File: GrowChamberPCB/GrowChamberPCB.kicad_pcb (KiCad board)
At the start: 4 copper layers, 100 x 100 mm, 194 parts, among them J1 Mister, J10 FoggerBasin, J11 TP, J12 Moisture Sensor 3, J13 Moisture Sensor 2, J14 UART, J15 FAE Fan, J16 DrainLevel, J17 TP, J18 TP, J19 TP, J2 Moisture Sensor 1, J20 TP, J21 TP, J22 TP, J23 TP, J24 TP, J25 TP, J26 TP, J27 TP, J28 TP, J29 TP, J3 SCD30, J30 TP, J31 TP, J32 TP, J33 TP, J34 TP, J35 TP, J36 TP, J37 TP, J38 TP, J39 TP, J4 Heater Fans, J40 TP, J41 TP, J42 TP, J43 TP, J44 TP, J45 TP, J47 Conn_01x04, J48 Conn_01x09, J49 TP, J5 Fogger Solenoid, J50 TP, J51 TP, J52 TP, J53 TP, J6 Drain Solenoid, J7 Water Solenoid, J8 Glycol Solenoid, J9 CircFan, P1 12V_In, P2 120V, P3 Screw Terminal, Q1 MOSFET, Q10 NPN, Q11 MOSFET, Q12 NPN, Q13 MOSFET, Q15 NPN, Q17 NPN, Q18 MOSFET, Q2 NPN, Q3 MOSFET, Q4 NPN, Q5 MOSFET, Q6 NPN, Q7 MOSFET, Q8 BRT30N70P3, Q9 NPN, SW1 Reset_Button_Internal, SW2 ResetButton_External, SW3 Bootmode_Internal, SW4 BootMode_External, U10 1N4007W, U11 AP63203WU-7, U12 1N4007W, U13 1N4007W, U14 1N4007W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

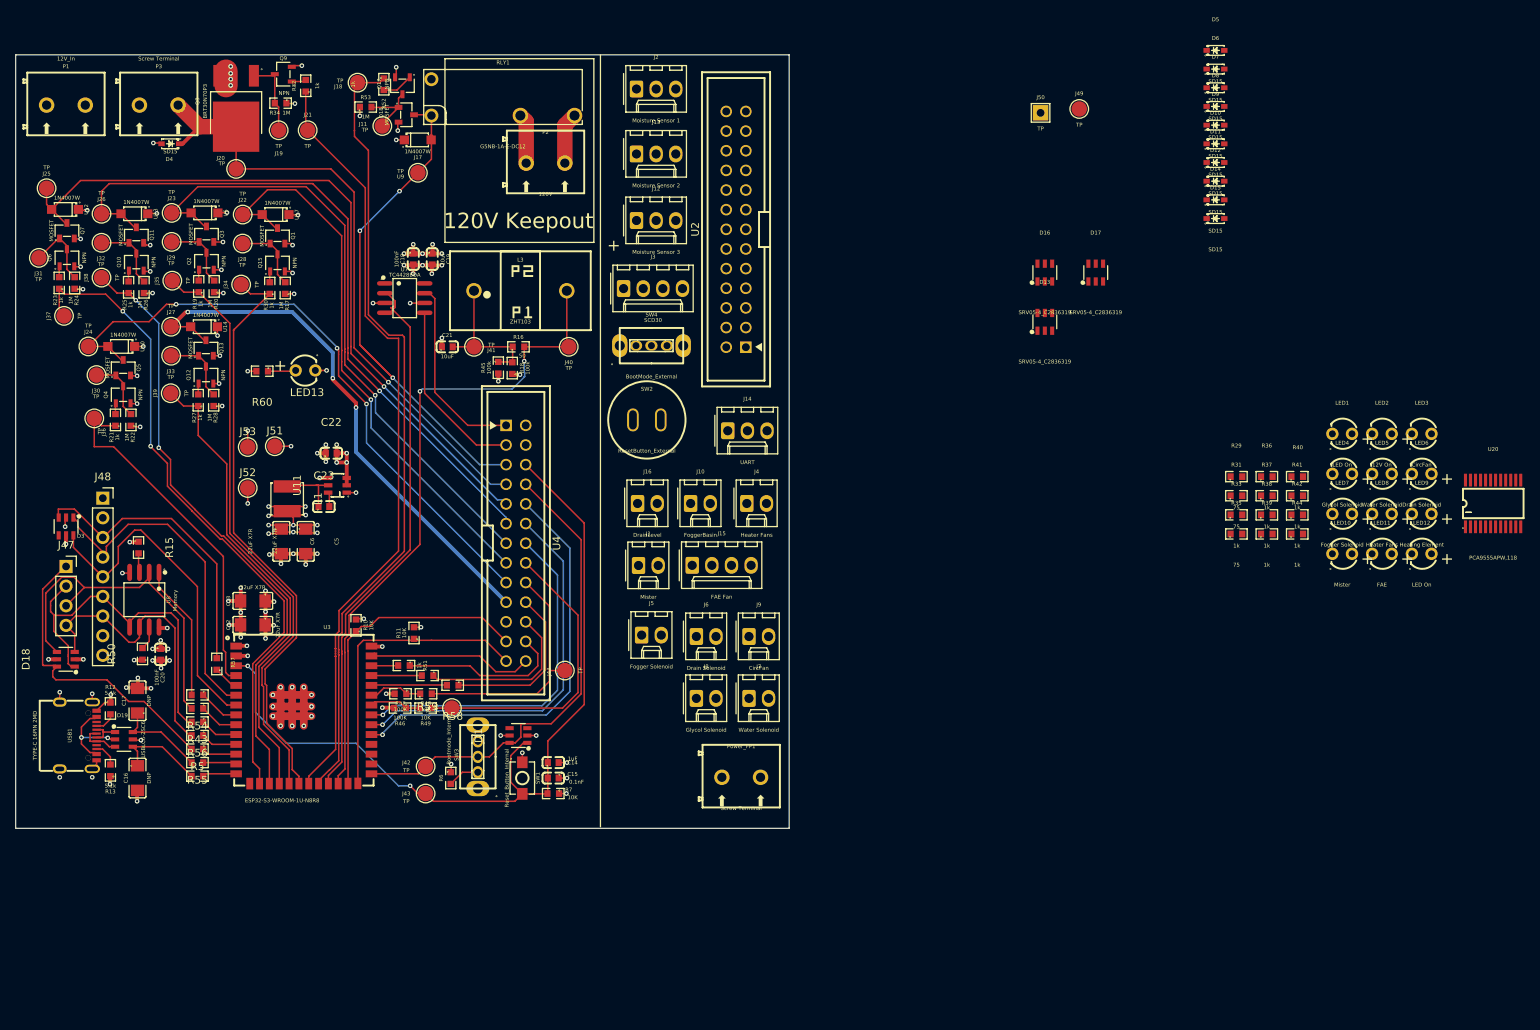
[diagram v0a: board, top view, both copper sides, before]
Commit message: finished routing
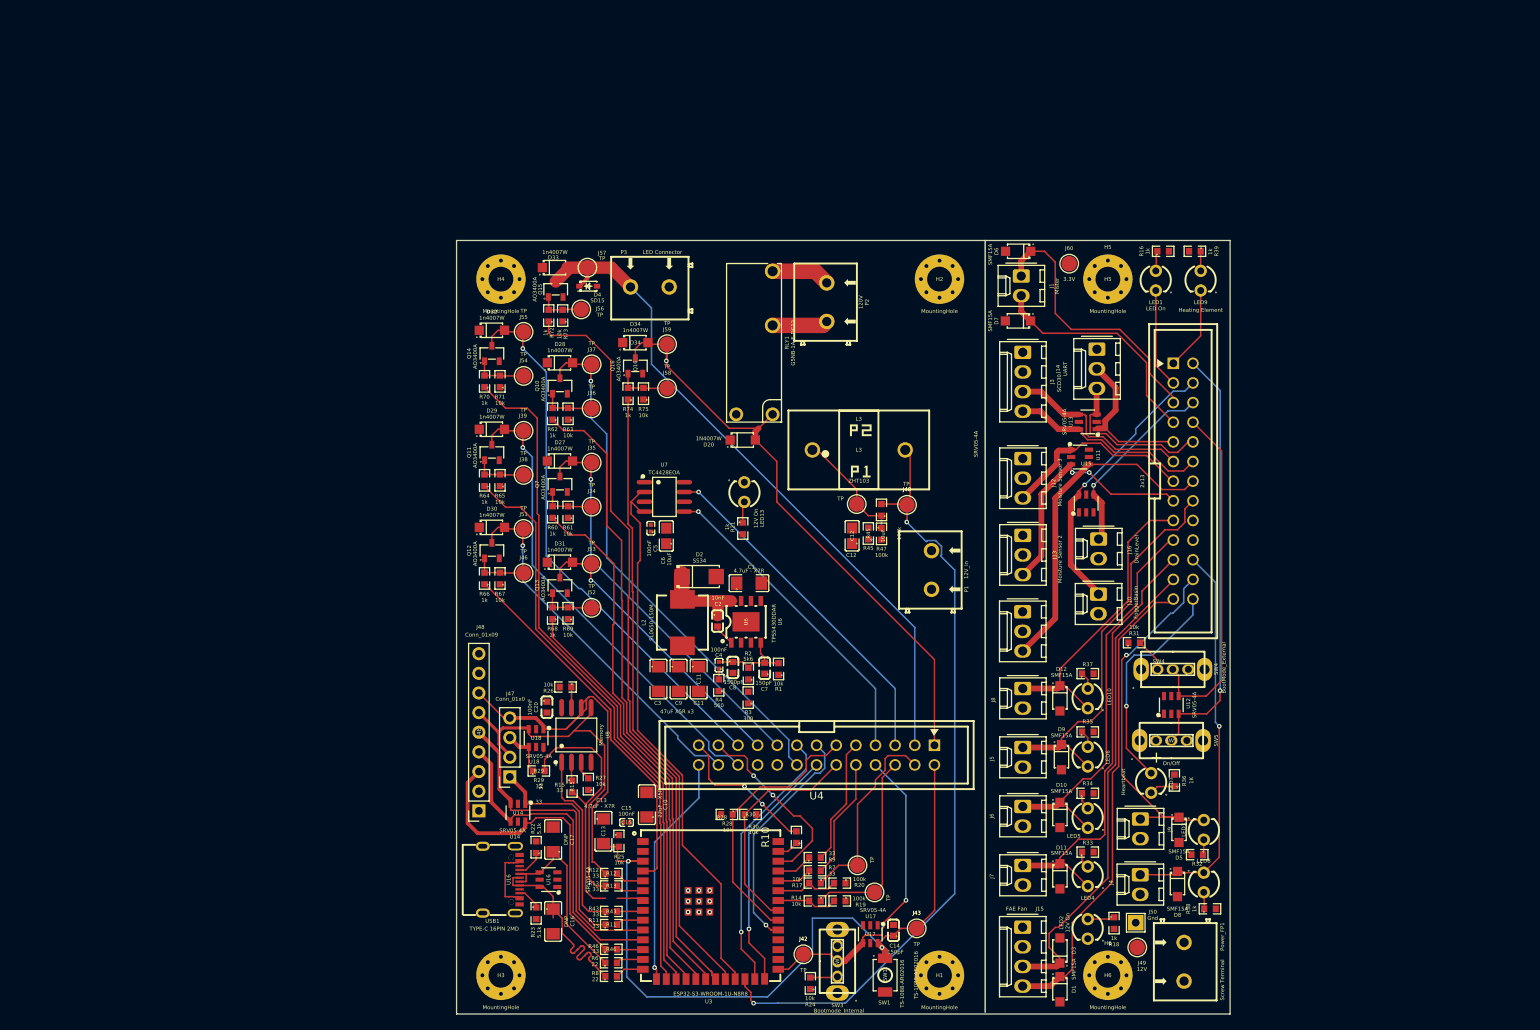
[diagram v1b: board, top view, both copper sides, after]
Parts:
- removed C18, C23: 100nF, easyeda2kicad:C0603
- removed C19, C21, C22: 10uF, easyeda2kicad:C0603
- removed D13, D16, D17, D18: SRV05-4_C2836319, easyeda2kicad:SOT-23-6_L2.9-W1.6-P0.95-LS2.8-BL
- removed D14, D15: SD15, easyeda2kicad:SOD-323_L1.7-W1.3-LS2.6-RD
- removed D19: USBLC6-2SC6, easyeda2kicad:SOT-23-6_L2.9-W1.6-P0.95-LS2.8-BL
- removed J11, J17, J18, J19, J20, J21, J22, J23, J24, J25, J26, J27, J28, J29, J30, J31, J32, J33: TP, TestPoint:TestPoint_Pad_D2.0mm
- removed L1: ANR4030T3R9M, easyeda2kicad:IND-SMD_L4.0-W4.0
- removed LED11: FAE, easyeda2kicad:LED-TH_BD3.9-P2.54-RD_RED
- removed LED12: LED On, easyeda2kicad:LED-TH_BD3.9-P2.54-RD_RED
- removed Q1, Q18, Q3, Q5: MOSFET, easyeda2kicad:SOT-23-3_L2.9-W1.3-P1.90-LS2.4-BR
- removed Q17, Q2, Q4, Q6, Q9: NPN, easyeda2kicad:SOT-23-3_L3.0-W1.7-P0.95-LS2.9-BR
- removed Q8: BRT30N70P3, easyeda2kicad:TO-252-2_L6.6-W6.1-P4.60-LS10.0-BR-CW
- removed R40, R41, R42, R44, R51, R52: 1k, easyeda2kicad:R0603
- removed R48, R49, R50: 10K, easyeda2kicad:R0603
- removed R53: 1M, easyeda2kicad:R0603
- removed R54, R55, R56, R57, R58, R59: 33, easyeda2kicad:R0603
- removed SW2: ResetButton_External, easyeda2kicad:CONN-TH_PB-05B-R
- removed U10, U5, U9: 1N4007W, easyeda2kicad:SOD-123FL_L2.7-W1.8-LS3.7-RD
- removed U20: PCA9555APW,118, easyeda2kicad:TSSOP-24_L7.8-W4.4-P0.65-LS6.4-BL
- added C1: 4.7uF - X7R, easyeda2kicad:C1206, F.Cu at (106.8, 80.3)
- added C10: 22uF - X5R, easyeda2kicad:C1206, F.Cu at (93.6, 108.9)
- added C11: 47uF X5R, easyeda2kicad:C1206, F.Cu at (100.3, 92.7)
- added C2: 10nF, easyeda2kicad:C0603, F.Cu at (102.7, 85.2)
- added C3: 47uF X5R, easyeda2kicad:C1206, F.Cu at (95.1, 92.7)
- added C4: 100nF, easyeda2kicad:C0402, F.Cu at (102.9, 90.9)
- added C7: 150pF, easyeda2kicad:C0603, F.Cu at (108.8, 91.3)
- added C8: 1500pF, easyeda2kicad:C0603, F.Cu at (104.7, 91.2)
- added C9: 47uF X5R, easyeda2kicad:C1206, F.Cu at (97.7, 92.7)
- added D2: SS34, easyeda2kicad:SMA_L4.3-W2.6-LS5.2-RD, F.Cu at (100.4, 79.5)
- added D20: 1N4007W, easyeda2kicad:SOD-123FL_L2.7-W1.8-LS3.8-RD, F.Cu at (106.0, 61.8)
- added D27: 1n4007W, easyeda2kicad:SOD-123FL_L2.7-W1.8-LS3.8-RD, F.Cu at (82.4, 64.5)
- added D28: 1n4007W, easyeda2kicad:SOD-123FL_L2.7-W1.8-LS3.8-RD, F.Cu at (82.4, 51.8)
- added D29: 1n4007W, easyeda2kicad:SOD-123FL_L2.7-W1.8-LS3.8-RD, F.Cu at (73.6, 60.4)
- added D30: 1n4007W, easyeda2kicad:SOD-123FL_L2.7-W1.8-LS3.8-RD, F.Cu at (73.6, 73.1)
- added D31: 1n4007W, easyeda2kicad:SOD-123FL_L2.7-W1.8-LS3.8-RD, F.Cu at (82.4, 77.6)
- added D32: 1n4007W, easyeda2kicad:SOD-123FL_L2.7-W1.8-LS3.8-RD, F.Cu at (73.6, 47.6)
- added D33: 1n4007W, easyeda2kicad:SOD-123FL_L2.7-W1.8-LS3.8-RD, F.Cu at (81.7, 39.5)
- added D34: 1n4007W, easyeda2kicad:SOD-123FL_L2.7-W1.8-LS3.8-RD, F.Cu at (92.1, 49.2)
- added H1: MountingHole, MountingHole:MountingHole_3.2mm_M3_Pad_Via, F.Cu at (131.4, 131.0)
- added H2: MountingHole, MountingHole:MountingHole_3.2mm_M3_Pad_Via, F.Cu at (131.4, 41.0)
- added H3: MountingHole, MountingHole:MountingHole_3.2mm_M3_Pad_Via, F.Cu at (74.7, 131.0)
- added H4: MountingHole, MountingHole:MountingHole_3.2mm_M3_Pad_Via, F.Cu at (74.7, 41.0)
- added H5: MountingHole, MountingHole:MountingHole_3.2mm_M3_Pad_Via, F.Cu at (153.2, 41.0)
- added H6: MountingHole, MountingHole:MountingHole_3.2mm_M3_Pad_Via, F.Cu at (153.2, 131.0)
- added J46: TP, TestPoint:TestPoint_Pad_D2.0mm, F.Cu at (77.7, 79.0)
- added J54: TP, TestPoint:TestPoint_Pad_D2.0mm, F.Cu at (77.7, 53.5)
- added J55: TP, TestPoint:TestPoint_Pad_D2.0mm, F.Cu at (77.7, 47.8)
- added J56: TP, TestPoint:TestPoint_Pad_D2.0mm, F.Cu at (85.1, 44.9)
- added J57: TP, TestPoint:TestPoint_Pad_D2.0mm, F.Cu at (85.9, 39.5)
- added J58: TP, TestPoint:TestPoint_Pad_D2.0mm, F.Cu at (96.2, 55.1)
- added J59: TP, TestPoint:TestPoint_Pad_D2.0mm, F.Cu at (96.2, 49.4)
- added J60: TP, TestPoint:TestPoint_Pad_D2.0mm, F.Cu at (148.2, 39.0)
- added L2: SL0650-150M, easyeda2kicad:IND-SMD_L7.0-W6.6, F.Cu at (98.2, 85.4)
- added Q14: AO3400A, easyeda2kicad:SOT-23-3_L2.9-W1.3-P1.90-LS2.4-BR, F.Cu at (73.6, 50.6)
- added Q16: AO3400A, easyeda2kicad:SOT-23-3_L2.9-W1.3-P1.90-LS2.4-BR, F.Cu at (92.1, 52.2)
- added R1: 10k, easyeda2kicad:R0603, F.Cu at (110.6, 91.4)
- added R14: 10k, easyeda2kicad:R0603, F.Cu at (115.3, 121.4)
- added R2: 5k6, easyeda2kicad:R0603, F.Cu at (106.7, 92.0)
- added R3: 300, easyeda2kicad:R0603, F.Cu at (106.7, 95.1)
- added R4: 560, easyeda2kicad:R0603, F.Cu at (102.9, 93.5)
- added R61: 10k, easyeda2kicad:R0603, F.Cu at (83.4, 71.1)
- added R62: 1k, easyeda2kicad:R0603, F.Cu at (81.4, 58.4)
- added R63: 10k, easyeda2kicad:R0603, F.Cu at (83.4, 58.4)
- added R64: 1k, easyeda2kicad:R0603, F.Cu at (72.6, 67.0)
- added R65: 10k, easyeda2kicad:R0603, F.Cu at (74.6, 67.0)
- added R66: 1k, easyeda2kicad:R0603, F.Cu at (72.6, 79.7)
- added R67: 10k, easyeda2kicad:R0603, F.Cu at (74.6, 79.7)
- added R68: 1k, easyeda2kicad:R0603, F.Cu at (81.4, 84.2)
- added R69: 10k, easyeda2kicad:R0603, F.Cu at (83.4, 84.2)
- added R70: 1k, easyeda2kicad:R0603, F.Cu at (72.6, 54.2)
- added R71: 10k, easyeda2kicad:R0603, F.Cu at (74.6, 54.2)
- added R72: 1k, easyeda2kicad:R0603, F.Cu at (80.9, 45.7)
- added R73: 10k, easyeda2kicad:R0603, F.Cu at (82.7, 45.7)
- added R74: 1k, easyeda2kicad:R0603, F.Cu at (91.2, 55.8)
- added R75: 10k, easyeda2kicad:R0603, F.Cu at (93.2, 55.8)
- added SW5: On/Off, easyeda2kicad:SW-TH_SS-12D02-VG4, F.Cu at (161.4, 100.7)
- added U15: SRV05-4A, easyeda2kicad:SOT-23-6_L2.9-W1.6-P0.95-LS2.9-BL, F.Cu at (150.4, 70.0)
- added U16: SRV05-4A, easyeda2kicad:SOT-23-6_L2.9-W1.6-P0.95-LS2.9-BL, F.Cu at (80.9, 118.6)
- added U18: SRV05-4A, easyeda2kicad:SOT-23-6_L2.9-W1.6-P0.95-LS2.9-BL, F.Cu at (79.3, 100.3)
- added U6: TPS5430DDAR, easyeda2kicad:ESOP-8_L4.9-W3.9-P1.27-LS6.0-TL-EP, F.Cu at (106.4, 85.3)
- C12, C6: value 22uF X7R -> 10uF; footprint easyeda2kicad:C1206 -> easyeda2kicad:C0805
- C13: value 22uF X7R -> 4.7uF - X7R
- C14: value 1uF -> 150pF
- C15: value 0.1nF -> 100nF; footprint easyeda2kicad:C0603 -> easyeda2kicad:C0402
- C5: value 22uF X7R -> 100nF; footprint easyeda2kicad:C1206 -> easyeda2kicad:C0402
- D1, D3: value SRV05-4_C2836319 -> SMF15A; footprint easyeda2kicad:SOT-23-6_L2.9-W1.6-P0.95-LS2.8-BL -> easyeda2kicad:SOD-123FL_L2.7-W1.8-LS3.8-RD
- D10, D11, D12, D5, D6, D7, D8, D9: value SD15 -> SMF15A; footprint easyeda2kicad:SOD-323_L1.7-W1.3-LS2.6-RD -> easyeda2kicad:SOD-123FL_L2.7-W1.8-LS3.8-RD
- J49: value TP -> 12V
- J50: value TP -> Gnd
- LED10: value Mister -> 12V On
- LED4: value Glycol Solenoid -> 12V On
- LED5: value Water Solenoid -> 12V On
- LED6: value Drain Solenoid -> 12V On
- LED7: value Fogger Solenoid -> 12V On
- P3: value Screw Terminal -> LED Connector
- Q10, Q12, Q15: value NPN -> AO3400A; footprint easyeda2kicad:SOT-23-3_L3.0-W1.7-P0.95-LS2.9-BR -> easyeda2kicad:SOT-23-3_L2.9-W1.3-P1.90-LS2.4-BR
- Q11, Q13, Q7: value MOSFET -> AO3400A
- R10: value 10K -> 1k
- R11, R15, R7: value 10K -> 33
- R12, R13: value 5.1k -> 33
- R16: value 50 -> 1k
- R17, R24, R26, R28: value 1M -> 10k
- R18: value 100k -> 1k
- R19: value 1k -> 100k
- R20: value 1M -> 100k
- R22: value 1M -> 5.1k
- R23: value 1k -> 5.1k
- R25, R27, R30: value 1k -> 10k
- R29: value 75 -> 33
- R31: value 75 -> 10k
- R34: value 1M -> 1k
- R35: value 75 -> 1k
- R36: value 1k -> 0603WAF750JT5E
- R46: value 100K -> 33
- R47: value 100K -> 100k
- R5: value 33 -> 50
- R6: value 10K -> 22
- R9: value 22 -> 33
- SW1: value Reset_Button_Internal -> TS-1088-AR02016; footprint easyeda2kicad:SW-SMD_L4.0-W2.9-LS5.0 -> easyeda2kicad:SW-SMD_L3.9-W3.0-P4.45
- U11: value AP63203WU-7 -> SRV05-4A; footprint easyeda2kicad:TSOT-26_L2.9-W1.6-P0.95-LS2.8-BL -> easyeda2kicad:SOT-23-6_L2.9-W1.6-P0.95-LS2.9-BL
- U12, U13, U14, U17: value 1N4007W -> SRV05-4A; footprint easyeda2kicad:SOD-123FL_L2.7-W1.8-LS3.7-RD -> easyeda2kicad:SOT-23-6_L2.9-W1.6-P0.95-LS2.9-BL
- U2: value ZX-IDC2.54-2-13PZZ -> 2x13
- moved U12 156.7 mm to (161.4, 96.0), turned to 0 degrees
- moved R32 152.2 mm to (164.8, 115.4), turned to 180 degrees
- moved D3 139.7 mm to (147.0, 127.8), turned to 90 degrees
- moved R34 137.3 mm to (150.6, 107.5), turned to 0 degrees
- moved R24 131.3 mm to (114.7, 132.0)
- moved P1 127.0 mm to (130.4, 78.6), turned to 90 degrees
- moved U13 126.2 mm to (150.6, 59.5), turned to 90 degrees
- moved U17 120.7 mm to (122.5, 125.7)
- moved R19 114.8 mm to (118.5, 121.4), turned to 180 degrees
- moved R20 111.8 mm to (118.5, 119.1), turned to 180 degrees
- moved J49 108.7 mm to (157.0, 127.4), turned to 180 degrees
- moved R18 105.8 mm to (154.0, 124.2), turned to -90 degrees
- moved J50 105.4 mm to (156.8, 124.2), turned to -90 degrees
- moved R17 103.0 mm to (115.3, 119.1), turned to 180 degrees
- moved R23 102.2 mm to (79.3, 123.0), turned to -90 degrees
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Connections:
- C12 pad 2: 3.3V -> Net-(J41-Pin_1)
- C13 pad 2: 3.3V -> EN
- C15 pad 1: GND -> 3.3V
- C15 pad 2: EN -> GND
- C16 pad 1: Out_D+ -> D+
- C17 pad 1: Out_D- -> D-
- C5 pad 1: 3.3V -> GND
- C5 pad 2: GND -> 12V
- C6 pad 1: 3.3V -> GND
- C6 pad 2: GND -> 12V
- D1 pad 1: EN -> External_Fan_PWM_FP
- D1 pad 2: GND -> GND_FP
- D10 pad 1: WaterSol_FP -> DrainSol_FP
- D11 pad 1: GlycolSol_FP -> FoggerSol_FP
- D12 pad 1: Piezo1_FP -> GlycolSol_FP
- D3 pad 1: Display_Reset -> Fan_Tach_FP
- D3 pad 2: GND -> GND_FP
- D7 pad 1: Heater Fans_FP -> Piezo1_FP
- D8 pad 1: FoggerSol_FP -> Heater Fans_FP
- D9 pad 1: DrainSol_FP -> WaterSol_FP
- J1 pad 1: Piezo1_FP -> Piezo2_FP
- J1 pad 2: Piezo2_FP -> Piezo1_FP
- J16 pad 1: 3.3V_FP -> Drain_Level_FP
- J16 pad 2: Drain_Level_FP -> 3.3V_FP
- J34 pad 1: HeaterFans_IO -> Net-(J34-Pin_1)
- J35 pad 1: FoggerSol_IO -> GlycolSol
- J36 pad 1: DrainSolIO -> Net-(J36-Pin_1)
- J37 pad 1: WaterSol_IO -> WaterSol
- J38 pad 1: GlycolSol_IO -> Net-(J38-Pin_1)
- J39 pad 1: CircFan_IO -> Heater Fans
- J47 pad 3: MISO -> MISO_ESD
- J5 pad 1: FoggerSol_FP -> WaterSol_FP
- J51 pad 1: GND -> Circ_Fan
- J52 pad 1: 3.3V -> Net-(J52-Pin_1)
- J53 pad 1: 12V -> DrainSol
- J7 pad 1: WaterSol_FP -> FoggerSol_FP
- LED10 pad 1: Net-(LED10-K) -> GlycolSol_FP
- LED4 pad 1: GlycolSol_FP -> FoggerSol_FP
- LED5 pad 1: WaterSol_FP -> DrainSol_FP
- LED6 pad 1: DrainSol_FP -> WaterSol_FP
- LED7 pad 1: FoggerSol_FP -> Net-(LED7-K)
- LED7 pad 2: Net-(LED7-A) -> Heartbeat_LED_FP
- Q10 pad 1: Net-(Q10-B) -> Net-(J36-Pin_1)
- Q10 pad 3: Net-(J32-Pin_1) -> WaterSol
- Q11 pad 1: Net-(J32-Pin_1) -> Net-(J38-Pin_1)
- Q11 pad 3: GlycolSol -> Heater Fans
- Q12 pad 1: Net-(Q12-B) -> Net-(J46-Pin_1)
- Q12 pad 3: Net-(J33-Pin_1) -> Circ_Fan
- Q13 pad 1: Net-(J33-Pin_1) -> Net-(J52-Pin_1)
- Q13 pad 3: Circ_Fan -> DrainSol
- Q15 pad 1: Net-(Q15-B) -> Net-(J56-Pin_1)
- Q15 pad 3: Net-(J28-Pin_1) -> LEDs
- Q7 pad 1: Net-(J31-Pin_1) -> Net-(J34-Pin_1)
- Q7 pad 3: WaterSol -> GlycolSol
- R10 pad 1: SDA -> Net-(U3-IO1)
- R10 pad 2: 3.3V -> External_Fan_PWM
- R11 pad 1: SCL -> CS_SD
- R11 pad 2: 3.3V -> Net-(U3-IO16)
- R12 pad 1: GND -> SCK
- R12 pad 2: Net-(USB1-CC1) -> Net-(U3-IO5)
- R13 pad 1: GND -> MOSI
- R13 pad 2: Net-(USB1-CC2) -> Net-(U3-IO6)
- R15 pad 1: 3.3V -> Net-(U8-DO)
- R15 pad 2: Net-(U8-IO2) -> MISO
- R16 pad 1: Net-(J41-Pin_1) -> Net-(LED1-A)
- R16 pad 2: KSD_Fault -> 12V_FP
- R17 pad 1: 12V -> Fogger_Basin_Float_Switch
- R17 pad 2: Net-(J28-Pin_1) -> FloatSwitch_IO
- R18 pad 1: 3.3V -> Net-(LED2-A)
- R18 pad 2: Net-(J41-Pin_1) -> 12V_FP
- R19 pad 1: FoggerSol_IO -> GND
- R19 pad 2: Net-(Q2-B) -> DrainLevel_IO
- R20 pad 1: 12V -> GND
- R20 pad 2: Net-(J29-Pin_1) -> FloatSwitch_IO
- R21 pad 1: DrainSolIO -> Net-(LED13-A)
- R21 pad 2: Net-(Q4-B) -> 12V
- R22 pad 1: 12V -> Net-(USB1-CC1)
- R22 pad 2: Net-(J30-Pin_1) -> GND
- R23 pad 1: WaterSol_IO -> Net-(USB1-CC2)
- R23 pad 2: Net-(Q6-B) -> GND
- R24 pad 1: 12V -> 3.3V
- R24 pad 2: Net-(J31-Pin_1) -> Net-(R24-Pad2)
- R25 pad 1: GlycolSol_IO -> 3.3V
- R25 pad 2: Net-(Q10-B) -> EN
- R26 pad 1: 12V -> Net-(U8-IO3)
- R26 pad 2: Net-(J32-Pin_1) -> 3.3V
- R27 pad 1: CircFan_IO -> 3.3V
- R27 pad 2: Net-(Q12-B) -> Net-(U8-IO2)
- R28 pad 1: 12V -> SCL
- R28 pad 2: Net-(J33-Pin_1) -> 3.3V
- R29 pad 1: Net-(LED10-A) -> MISO_ESD
- R29 pad 2: 3.3V_FP -> MISO
- R30 pad 1: HeaterFans_IO -> SDA
- R30 pad 2: Net-(Q15-B) -> 3.3V
- R31 pad 1: Net-(LED12-A) -> 3.3V
- R31 pad 2: 3.3V_FP -> Net-(R31-Pad2)
- R32 pad 1: LEDIO -> Net-(LED3-A)
- R32 pad 2: Net-(Q9-B) -> 12V_FP
- R33 pad 1: Net-(LED3-A) -> Net-(LED4-A)
- R34 pad 1: 12V -> Net-(LED5-A)
- R34 pad 2: Net-(J19-Pin_1) -> 12V_FP
- R35 pad 1: Net-(LED11-A) -> Net-(LED6-A)
- R35 pad 2: 3.3V_FP -> 12V_FP
- R36 pad 1: Net-(LED4-A) -> Net-(LED7-K)
- R36 pad 2: 12V_FP -> GND_FP
- R37 pad 1: Net-(LED5-A) -> Net-(LED10-A)
- R38 pad 1: Net-(LED6-A) -> Net-(LED8-A)
- R39 pad 1: Net-(LED7-A) -> Net-(LED9-A)
- R43 pad 1: Net-(U3-IO16) -> CS_Memory
- R43 pad 2: MISO -> Net-(U3-IO15)
- R45 pad 1: Net-(J41-Pin_1) -> GND
- R45 pad 2: GND -> Net-(J41-Pin_1)
- R46 pad 1: DrainLevel_IO -> CS_Display
- R46 pad 2: GND -> Net-(U3-IO8)
- R47 pad 1: FloatSwitch_IO -> Net-(J41-Pin_1)
- R47 pad 2: GND -> 3.3V
- R5 pad 1: Net-(U3-IO18) -> Net-(J41-Pin_1)
- R5 pad 2: SCK -> KSD_Fault
- R6 pad 1: 3.3V -> D-
- R6 pad 2: Net-(R6-Pad2) -> IO19
- R60 pad 1: Net-(LED13-A) -> GlycolSol_IO
- R60 pad 2: 12V -> Net-(J34-Pin_1)
- R7 pad 1: 3.3V -> Net-(U3-RXD0)
- R7 pad 2: EN -> RXD0
- R8 pad 1: Out_D- -> D+
- R8 pad 2: IO19 -> IO20
- R9 pad 1: Out_D+ -> Net-(U3-TXD0)
- R9 pad 2: IO20 -> TXD0
- SW3 pad 1: Net-(R6-Pad2) -> Net-(R24-Pad2)
- SW4 pad 1: unconnected-(SW4-Pad1) -> Net-(R31-Pad2)
- U11 pad 1: 3.3V -> SoilMoisture4_FP
- U11 pad 2: 12V -> GND_FP
- U11 pad 3: 12V -> SoilMoisture2_FP
- U11 pad 4: GND -> SoilMoisture1_FP
- U11 pad 5: Net-(U11-SW) -> 3.3V_FP
- U11 pad 6: Net-(U11-BST) -> /Faceplate/3.3V ESD/IO3
- U12 pad 1: 12V -> /Faceplate/Data Line ESD/IO1
- U12 pad 2: WaterSol -> GND_FP
- U13 pad 1: 12V -> TXD0_FP
- U13 pad 2: GlycolSol -> GND_FP
- U14 pad 1: 12V -> CS_SD
- U14 pad 2: Circ_Fan -> GND_FP
- U17 pad 1: 12V -> /ESP32/Data Line ESD3/IO1
- U17 pad 2: Heater Fans -> GND_FP
- U2 pad 1: Piezo2_FP -> Heater_ON_FP
- U2 pad 10: SoilMoisture4_FP -> RXD0_FP
- U2 pad 11: GlycolSol_FP -> SCL_FP
- U2 pad 12: SoilMoisture2_FP -> SDA_FP
- U2 pad 13: FoggerSol_FP -> SoilMoisture4_FP
- U2 pad 15: Heater Fans_FP -> SoilMoisture2_FP
- U2 pad 16: Drain_Level_FP -> WaterSol_FP
- U2 pad 17: DrainSol_FP -> GlycolSol_FP
- U2 pad 18: Fogger_Basin_Float_Switch_FP -> 3.3V_FP
- U2 pad 19: Circ_Fan_FP -> DrainSol_FP
- U2 pad 2: 3.3V_FP -> EN_FP
- U2 pad 20: RXD0_FP -> 3.3V_FP
- U2 pad 21: unconnected-(U2-Pad21) -> FoggerSol_FP
- U2 pad 22: TXD0_FP -> Heater Fans_FP
- U2 pad 23: SDA_FP -> Fan_Tach_FP
- U2 pad 24: External_Fan_PWM_FP -> Circ_Fan_FP
- U2 pad 25: SCL_FP -> External_Fan_PWM_FP
- U2 pad 26: Fan_Tach_FP -> Heartbeat_LED_FP
- U2 pad 3: Piezo1_FP -> LEDs_FP
- U2 pad 4: 3.3V_FP -> Fogger_Basin_Float_Switch_FP
- U2 pad 5: Heater_ON_FP -> Piezo2_FP
- U2 pad 6: EN_FP -> Drain_Level_FP
- U2 pad 7: LEDs_FP -> Piezo1_FP
- U2 pad 9: WaterSol_FP -> TXD0_FP
- U3 pad 10: Net-(U3-IO17) -> DC_Display
- U3 pad 11: Net-(U3-IO18) -> Display_Reset
- U3 pad 15: unconnected-(U3-IO3-Pad15) -> Heartbeat_LED
- U3 pad 16: WaterSol_IO -> HeaterFans_IO
- U3 pad 17: GlycolSol_IO -> FoggerSol_IO
- U3 pad 18: CircFan_IO -> DrainSolIO
- U3 pad 19: FoggerSol_IO -> GlycolSol_IO
- U3 pad 20: HeaterFans_IO -> WaterSol_IO
- U3 pad 25: SDA -> Soil_Moisture2
- U3 pad 26: SCL -> Soil_Moisture1
- U3 pad 32: Soil_Moisture2 -> SCL
- U3 pad 33: Soil_Moisture1 -> SDA
- U3 pad 38: Net-(U3-IO2) -> Fan_Tach
- U3 pad 39: Fan_Tach -> Net-(U3-IO1)
- U3 pad 4: DrainSolIO -> CircFan_IO
- U3 pad 6: Display_Reset -> Net-(U3-IO6)
- U3 pad 7: DC_Display -> MISO
- U4 pad 1: Piezo2 -> Heater_ON
- U4 pad 10: Soil_Moisture4 -> RXD0
- U4 pad 11: GlycolSol -> SCL
- U4 pad 12: Soil_Moisture2 -> SDA
- U4 pad 13: FoggerSol -> Soil_Moisture4
- U4 pad 15: Heater Fans -> Soil_Moisture2
- U4 pad 16: Drain_Level -> WaterSol
- U4 pad 17: DrainSol -> GlycolSol
- U4 pad 18: Fogger_Basin_Float_Switch -> 3.3V
- U4 pad 19: Circ_Fan -> DrainSol
- U4 pad 2: 3.3V -> EN
- U4 pad 20: RXD0 -> 3.3V
- U4 pad 21: unconnected-(U4-Pad21) -> FoggerSol
- U4 pad 22: TXD0 -> Heater Fans
- U4 pad 23: SDA -> Fan_Tach
- U4 pad 24: External_Fan_PWM -> Circ_Fan
- U4 pad 25: SCL -> External_Fan_PWM
- U4 pad 26: Fan_Tach -> Heartbeat_LED
- U4 pad 3: Piezo1 -> LEDs
- U4 pad 4: 3.3V -> Fogger_Basin_Float_Switch
- U4 pad 5: Heater_ON -> Piezo2
- U4 pad 6: EN -> Drain_Level
- U4 pad 7: LEDs -> Piezo1
- U4 pad 9: WaterSol -> TXD0
- U8 pad 2: MISO -> Net-(U8-DO)
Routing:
- net GND: track 112.3 -> 0.00 mm, vias 81 -> 9
- net Fan_Tach_FP: track 0.00 -> 62.1 mm
- net External_Fan_PWM_FP: track 0.00 -> 61.6 mm
- net FoggerSol_FP: track 0.00 -> 56.9 mm
- net EN_FP: track 0.00 -> 55.0 mm, vias 0 -> 1
- net Heater Fans_FP: track 0.00 -> 51.9 mm, vias 0 -> 1
- net DrainSol_FP: track 0.00 -> 51.1 mm
- net 3.3V: track 50.8 -> 0.00 mm, vias 32 -> 0
- net WaterSol_FP: track 0.00 -> 50.2 mm
- net Circ_Fan_FP: track 0.00 -> 47.6 mm, vias 0 -> 1
- net BootMode_FP: track 0.00 -> 45.1 mm
- net 12V: track 44.0 -> 0.00 mm, vias 27 -> 0
- net DrainSol: track 81.4 -> 37.9 mm, vias 3 -> 1
- net SoilMoisture1_FP: track 0.00 -> 42.9 mm
- net GlycolSol_FP: track 0.00 -> 39.0 mm
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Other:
- board text added: "1K"
- board text added: "3.3V"
- board text added: "33"
- board text added: "47uF X5R x3"
- board text added: "Conn_01x0"
- board text added: "Heartbeat"
- board text added: "J39"
- board text added: "TS-1088-AR02016"
- board text removed: "120V Keepout"
